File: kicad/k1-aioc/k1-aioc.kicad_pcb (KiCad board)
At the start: 2 copper layers, 47.5 x 80 mm, 58 parts, among them J1 12401832E402A, J2 Conn_01x07_Male, J3 AUDIO, J4 CAT, Q1 PZT2222A, Q2 PZT2222A, U1 TLV1117LV-33, U2 STM32F373CBTx, U3 TLV1117LV-33, U4 CRE1S0505SC, U5 ADUM3160, Y1 8MHz/20pF

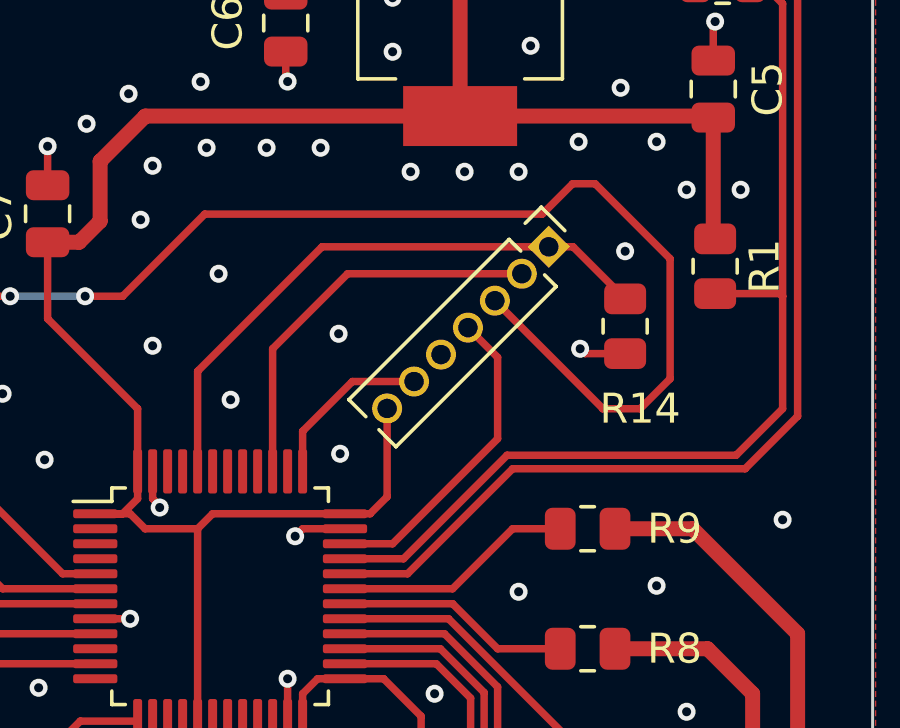
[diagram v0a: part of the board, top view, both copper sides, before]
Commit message: Silk Screen artwork on pcb back
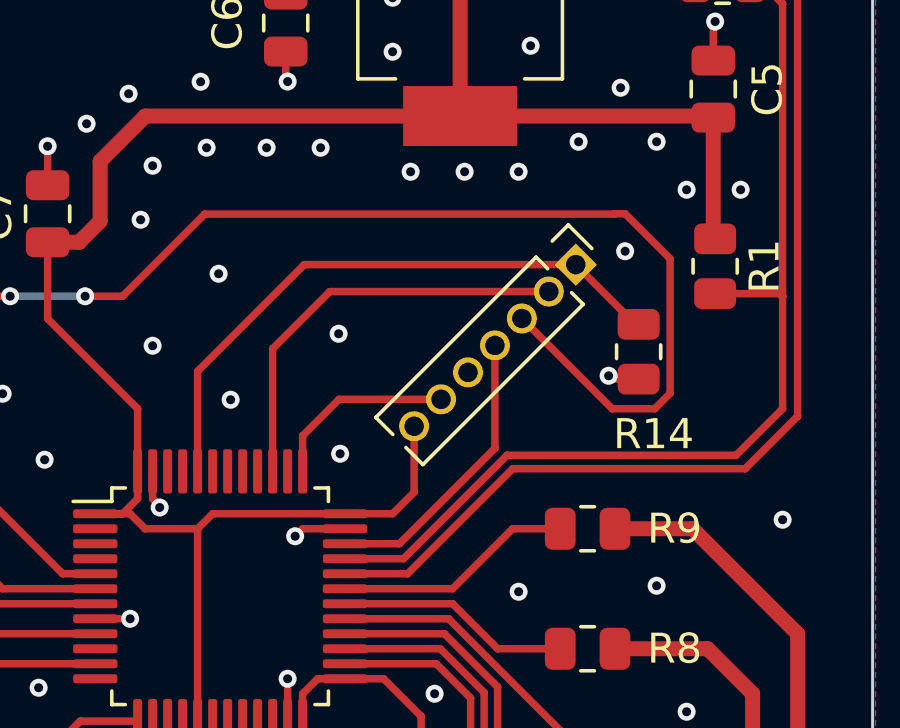
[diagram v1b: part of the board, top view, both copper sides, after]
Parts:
- added G***: LOGO, symbols:hb9uf_logo, B.Cu at (234.2, 62.6)
- added SYM: Symbol_OSHW-Logo_SilkScreen_07Jul2012, symbols:Symbol_OSHW-Logo_SilkScreen, B.Cu at (244.2, 83.0)
- moved J2 1.08 mm to (241.1, 68.7)
- moved R14 0.96 mm to (243.2, 71.6)
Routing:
- net /NRST: track 75.9 -> 74.2 mm
- net /SWDIO: track 10.7 -> 9.74 mm
- net /SWO: track 13.4 -> 14.1 mm
- net /SWCLK: track 5.74 -> 6.31 mm
- net GND: track 38.8 -> 38.2 mm
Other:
- board text added: "All-In-One-Box"
- board text added: "By Matt Weyland (HB9FRV) based on work by skuep Rev 1.0, (c) 2024, MIT License"
- board text added: "HB9UF HB9UHF"
